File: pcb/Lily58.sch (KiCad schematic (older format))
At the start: 130 parts, among them J2 4PIN, J3 Conn_01x06_Female, J4 Conn_01x06_Female, P1 i2c_pin, P2 i2c_pin, SW1 SW_PUSH, SW10 SW_PUSH, SW11 SW_PUSH, SW12 SW_PUSH, SW13 SW_PUSH, SW14 SW_PUSH, SW15 SW_PUSH, SW16 SW_PUSH, SW17 SW_PUSH, SW18 SW_PUSH, SW19 SW_PUSH, SW2 SW_PUSH, SW20 SW_PUSH, SW21 SW_PUSH, SW22 SW_PUSH, SW23 SW_PUSH, SW24 SW_PUSH, SW25 SW_PUSH, SW26 SW_PUSH, SW27 SW_PUSH, SW28 SW_PUSH, SW29 SW_PUSH, SW3 SW_PUSH, SW4 SW_PUSH, SW5 SW_PUSH, SW6 SW_PUSH, SW7 SW_PUSH, SW8 SW_PUSH, SW9 SW_PUSH, U1 ProMicro

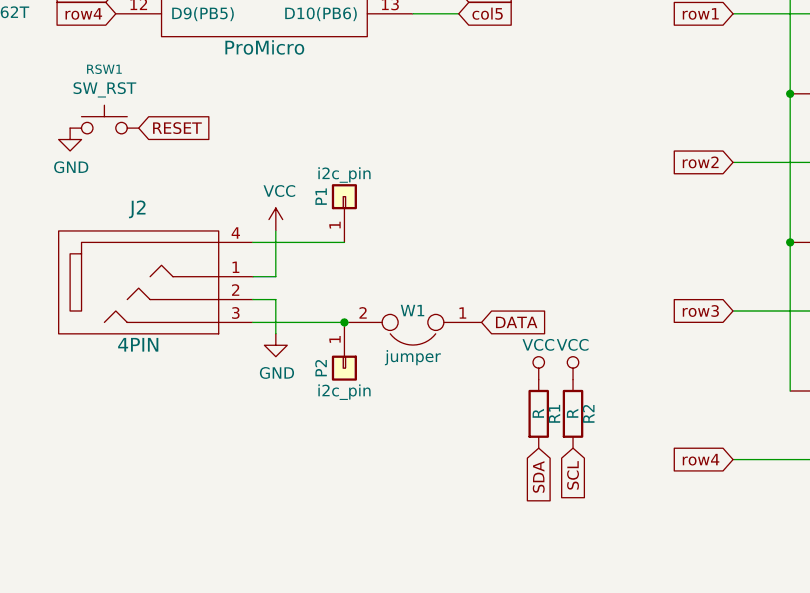
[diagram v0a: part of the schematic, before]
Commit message: change 3.5mm jack assign
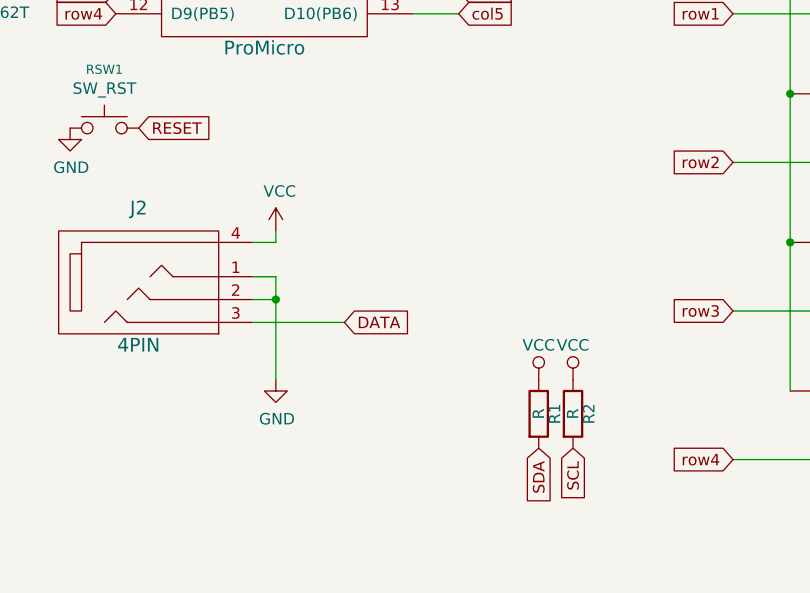
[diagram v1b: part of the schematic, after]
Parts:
- removed P1, P2: i2c_pin, Lily58-footprint:1pin_conn, symbol Lily58-rescue:i2c_pin-Lily58-cache
- removed W1: jumper, Lily58-footprint:jumper_data, symbol Device:Jumper
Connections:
- net DATA: now also J2.3
- net GND: now also J2.1
- net VCC: now also J2.4; no longer J2.1
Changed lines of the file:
@@
 $EndDescr
-$Comp
-L Lily58-rescue:ProMicro_2-Lily58-cache U1
-U 1 1 5B722440
-P 3200 2650
-F 0 "U1" H 3200 3350 60  0000 C CNN
-F 1 "ProMicro" H 3200 1950 60  0000 C CNN
-F 2 "Lily58-footprint:ProMicro_rev2" H 3300 1600 60  0001 C CNN
-F 3 "" H 3300 1600 60  0000 C CNN
-	1    3200 2650
-	1    0    0    -1
-$EndComp
 $Comp
 L Lily58-rescue:SW_PUSH-Lily58-cache SW25
@@
 Wire Wire Line
 	2550 2400 2300 2400
-Connection ~ 2550 2400
 $Comp
 L power:GND #PWR02
 U 1 1 5B8F3218
-P 3250 4600
-F 0 "#PWR02" H 3250 4350 50  0001 C CNN
-F 1 "GND" H 3255 4427 50  0000 C CNN
-F 2 "" H 3250 4600 50  0001 C CNN
-F 3 "" H 3250 4600 50  0001 C CNN
-	1    3250 4600
+P 3250 4800
+F 0 "#PWR02" H 3250 4550 50  0001 C CNN
+F 1 "GND" H 3255 4627 50  0000 C CNN
+F 2 "" H 3250 4800 50  0001 C CNN
+F 3 "" H 3250 4800 50  0001 C CNN
+	1    3250 4800
 	1    0    0    -1
 $EndComp
@@
 	1    0    0    -1
 $EndComp
-Wire Wire Line
-	3250 4350 3150 4350
-Wire Wire Line
-	3150 4450 3250 4450
-$Comp
-L Lily58-rescue:i2c_pin-Lily58-cache P1
-U 1 1 5B8F6780
-P 3550 4000
-F 0 "P1" H 3550 4100 50  0000 C CNN
-F 1 "i2c_pin" V 3650 4000 50  0000 C CNN
-F 2 "Lily58-footprint:1pin_conn" H 3550 4000 50  0001 C CNN
-F 3 "" H 3550 4000 50  0001 C CNN
-	1    3550 4000
-	0    -1   -1   0
-$EndComp
-$Comp
-L Lily58-rescue:i2c_pin-Lily58-cache P2
-U 1 1 5B8F6980
-P 3550 4750
-F 0 "P2" H 3550 4650 50  0000 C CNN
-F 1 "i2c_pin" V 3650 4750 50  0000 C CNN
-F 2 "Lily58-footprint:1pin_conn" H 3550 4750 50  0001 C CNN
-F 3 "" H 3550 4750 50  0001 C CNN
-	1    3550 4750
-	0    1    1    0
-$EndComp
-Wire Wire Line
-	3150 4550 3550 4550
-Wire Wire Line
-	3150 4200 3550 4200
-Wire Wire Line
-	3250 4150 3250 4350
-Wire Wire Line
-	3250 4450 3250 4600
-$Comp
-L Device:Jumper W1
-U 1 1 5B900157
-P 3850 4550
-F 0 "W1" H 3850 4500 50  0000 C CNN
-F 1 "jumper" H 3850 4700 50  0000 C CNN
-F 2 "Lily58-footprint:jumper_data" H 3850 4550 50  0001 C CNN
-F 3 "" H 3850 4550 50  0000 C CNN
-	1    3850 4550
-	-1   0    0    1
-$EndComp
 Text GLabel 2550 2200 0    50   Input ~ 0
 DATA
-Text GLabel 4150 4550 2    50   Input ~ 0
+Text GLabel 3550 4550 2    50   Input ~ 0
 DATA
-Connection ~ 3550 4550
 Text Label 3850 3000 0    50   ~ 0
 MISO
@@
 Wire Wire Line
 	1850 2700 1850 2750
-Wire Wire Line
-	1850 2700 2550 2700
 Connection ~ 1850 2700
 $Comp
@@
 Wire Wire Line
 	8400 10800 9800 10800
+Wire Wire Line
+	3150 4200 3250 4200
+Wire Wire Line
+	3250 4200 3250 4150
+Wire Wire Line
+	3150 4350 3250 4350
+Wire Wire Line
+	3250 4350 3250 4450
+Wire Wire Line
+	3150 4450 3250 4450
+Connection ~ 3250 4450
+Wire Wire Line
+	3250 4450 3250 4800
+Wire Wire Line
+	3550 4550 3150 4550
+Connection ~ 2550 2400
+Wire Wire Line
+	1850 2700 2550 2700
+$Comp
+L Lily58-rescue:ProMicro_2-Lily58-cache U1
+U 1 1 5B722440
+P 3200 2650
+F 0 "U1" H 3200 3350 60  0000 C CNN
+F 1 "ProMicro" H 3200 1950 60  0000 C CNN
+F 2 "Lily58-footprint:ProMicro_rev2" H 3300 1600 60  0001 C CNN
+F 3 "" H 3300 1600 60  0000 C CNN
+	1    3200 2650
+	1    0    0    -1
+$EndComp
 $EndSCHEMATC

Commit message: Revert "change 3.5mm jack assign"
This reverts commit aa684eaece7f45b972ff72976500a763c7363c79.
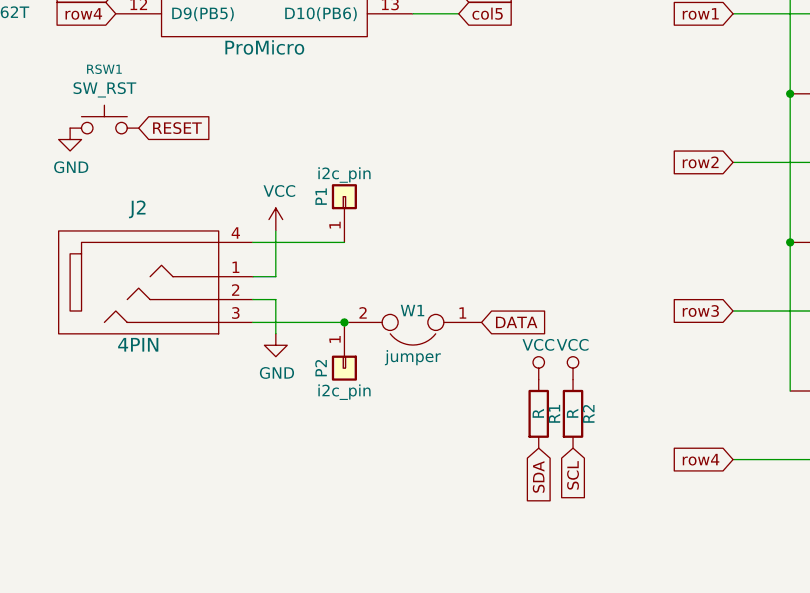
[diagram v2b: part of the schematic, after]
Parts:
- added P1, P2: i2c_pin, Lily58-footprint:1pin_conn, symbol Lily58-rescue:i2c_pin-Lily58-cache
- added W1: jumper, Lily58-footprint:jumper_data, symbol Device:Jumper
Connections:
- net DATA: now also W1.1; no longer J2.3
- net GND: no longer J2.1
- net VCC: now also J2.1; no longer J2.4
- new net: J2.3, P2.1 (Pin_1), W1.2
- new net: J2.4, P1.1 (Pin_1)
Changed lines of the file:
@@
 $EndDescr
+$Comp
+L Lily58-rescue:ProMicro_2-Lily58-cache U1
+U 1 1 5B722440
+P 3200 2650
+F 0 "U1" H 3200 3350 60  0000 C CNN
+F 1 "ProMicro" H 3200 1950 60  0000 C CNN
+F 2 "Lily58-footprint:ProMicro_rev2" H 3300 1600 60  0001 C CNN
+F 3 "" H 3300 1600 60  0000 C CNN
+	1    3200 2650
+	1    0    0    -1
+$EndComp
 $Comp
 L Lily58-rescue:SW_PUSH-Lily58-cache SW25
@@
 Wire Wire Line
 	2550 2400 2300 2400
+Connection ~ 2550 2400
 $Comp
 L power:GND #PWR02
 U 1 1 5B8F3218
-P 3250 4800
-F 0 "#PWR02" H 3250 4550 50  0001 C CNN
-F 1 "GND" H 3255 4627 50  0000 C CNN
-F 2 "" H 3250 4800 50  0001 C CNN
-F 3 "" H 3250 4800 50  0001 C CNN
-	1    3250 4800
+P 3250 4600
+F 0 "#PWR02" H 3250 4350 50  0001 C CNN
+F 1 "GND" H 3255 4427 50  0000 C CNN
+F 2 "" H 3250 4600 50  0001 C CNN
+F 3 "" H 3250 4600 50  0001 C CNN
+	1    3250 4600
 	1    0    0    -1
 $EndComp
@@
 	1    0    0    -1
 $EndComp
+Wire Wire Line
+	3250 4350 3150 4350
+Wire Wire Line
+	3150 4450 3250 4450
+$Comp
+L Lily58-rescue:i2c_pin-Lily58-cache P1
+U 1 1 5B8F6780
+P 3550 4000
+F 0 "P1" H 3550 4100 50  0000 C CNN
+F 1 "i2c_pin" V 3650 4000 50  0000 C CNN
+F 2 "Lily58-footprint:1pin_conn" H 3550 4000 50  0001 C CNN
+F 3 "" H 3550 4000 50  0001 C CNN
+	1    3550 4000
+	0    -1   -1   0
+$EndComp
+$Comp
+L Lily58-rescue:i2c_pin-Lily58-cache P2
+U 1 1 5B8F6980
+P 3550 4750
+F 0 "P2" H 3550 4650 50  0000 C CNN
+F 1 "i2c_pin" V 3650 4750 50  0000 C CNN
+F 2 "Lily58-footprint:1pin_conn" H 3550 4750 50  0001 C CNN
+F 3 "" H 3550 4750 50  0001 C CNN
+	1    3550 4750
+	0    1    1    0
+$EndComp
+Wire Wire Line
+	3150 4550 3550 4550
+Wire Wire Line
+	3150 4200 3550 4200
+Wire Wire Line
+	3250 4150 3250 4350
+Wire Wire Line
+	3250 4450 3250 4600
+$Comp
+L Device:Jumper W1
+U 1 1 5B900157
+P 3850 4550
+F 0 "W1" H 3850 4500 50  0000 C CNN
+F 1 "jumper" H 3850 4700 50  0000 C CNN
+F 2 "Lily58-footprint:jumper_data" H 3850 4550 50  0001 C CNN
+F 3 "" H 3850 4550 50  0000 C CNN
+	1    3850 4550
+	-1   0    0    1
+$EndComp
 Text GLabel 2550 2200 0    50   Input ~ 0
 DATA
-Text GLabel 3550 4550 2    50   Input ~ 0
+Text GLabel 4150 4550 2    50   Input ~ 0
 DATA
+Connection ~ 3550 4550
 Text Label 3850 3000 0    50   ~ 0
 MISO
@@
 Wire Wire Line
 	1850 2700 1850 2750
+Wire Wire Line
+	1850 2700 2550 2700
 Connection ~ 1850 2700
 $Comp
@@
 Wire Wire Line
 	8400 10800 9800 10800
-Wire Wire Line
-	3150 4200 3250 4200
-Wire Wire Line
-	3250 4200 3250 4150
-Wire Wire Line
-	3150 4350 3250 4350
-Wire Wire Line
-	3250 4350 3250 4450
-Wire Wire Line
-	3150 4450 3250 4450
-Connection ~ 3250 4450
-Wire Wire Line
-	3250 4450 3250 4800
-Wire Wire Line
-	3550 4550 3150 4550
-Connection ~ 2550 2400
-Wire Wire Line
-	1850 2700 2550 2700
-$Comp
-L Lily58-rescue:ProMicro_2-Lily58-cache U1
-U 1 1 5B722440
-P 3200 2650
-F 0 "U1" H 3200 3350 60  0000 C CNN
-F 1 "ProMicro" H 3200 1950 60  0000 C CNN
-F 2 "Lily58-footprint:ProMicro_rev2" H 3300 1600 60  0001 C CNN
-F 3 "" H 3300 1600 60  0000 C CNN
-	1    3200 2650
-	1    0    0    -1
-$EndComp
 $EndSCHEMATC
